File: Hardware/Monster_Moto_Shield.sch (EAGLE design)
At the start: 44 parts, among them Q1 FDD8580, Q2 FDD8580, U1 VNH2SP30, U2 VNH2SP30, U3 ARDUINO_SHIELDLABEL

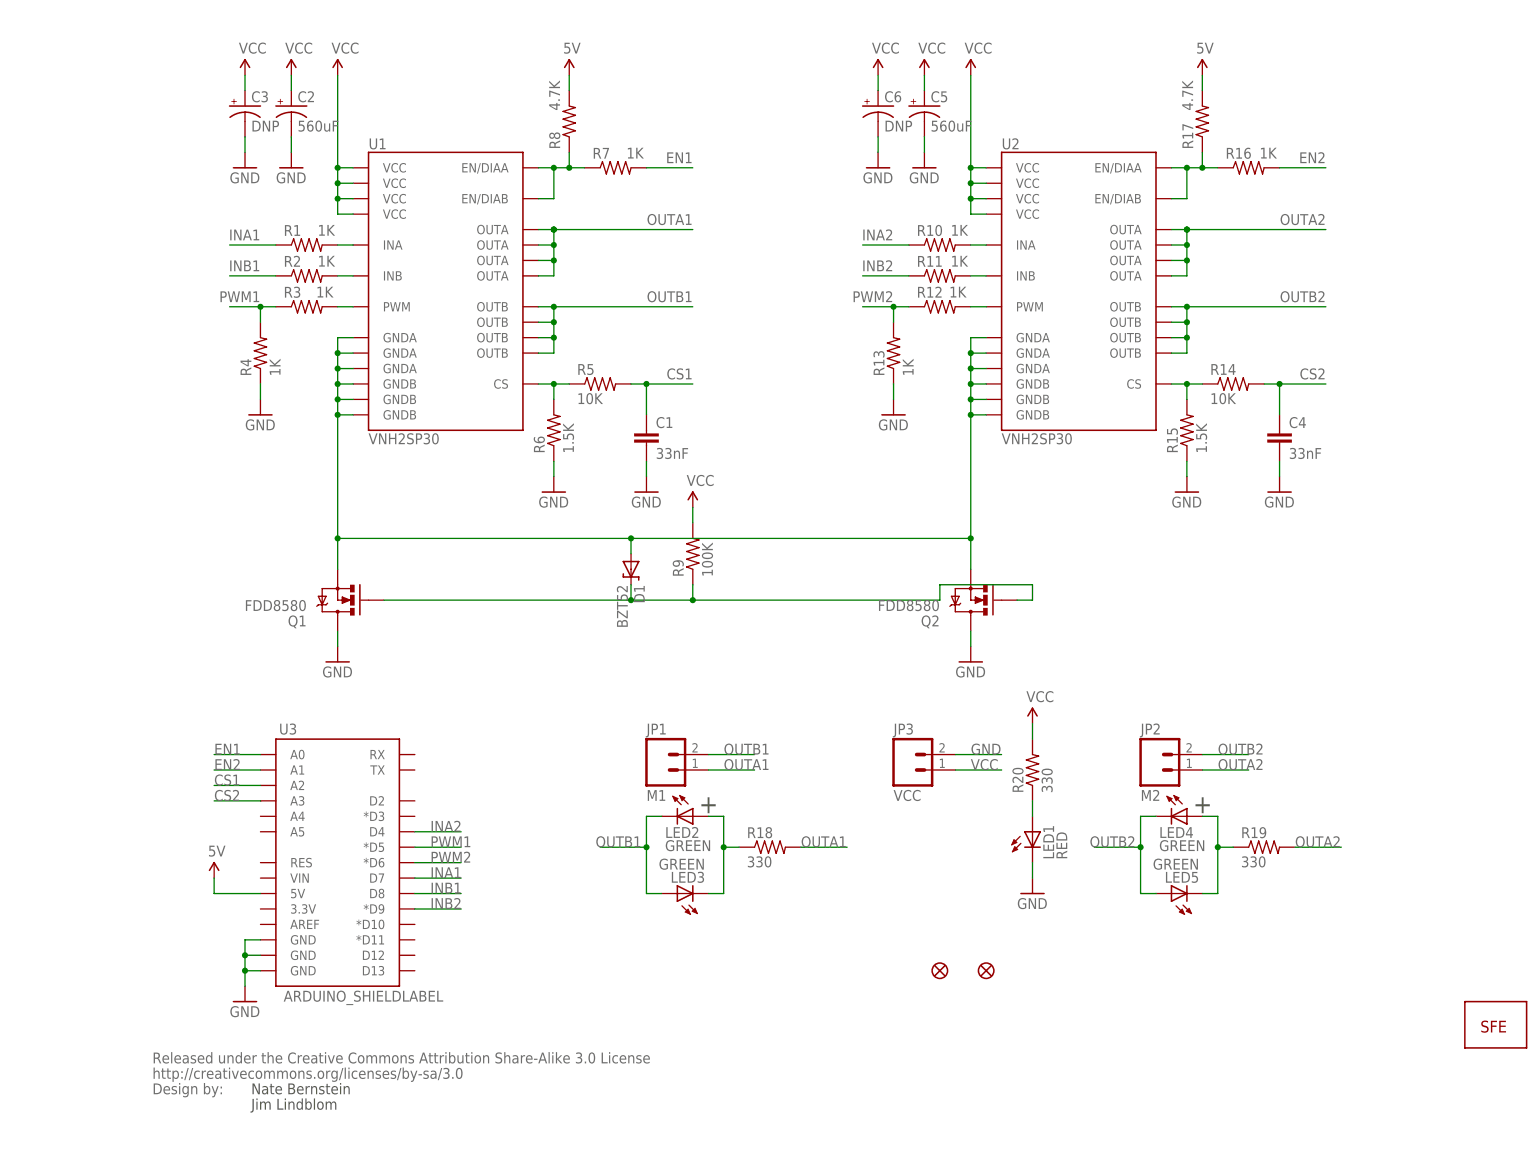
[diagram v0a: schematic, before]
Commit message: Commit bec of computer change
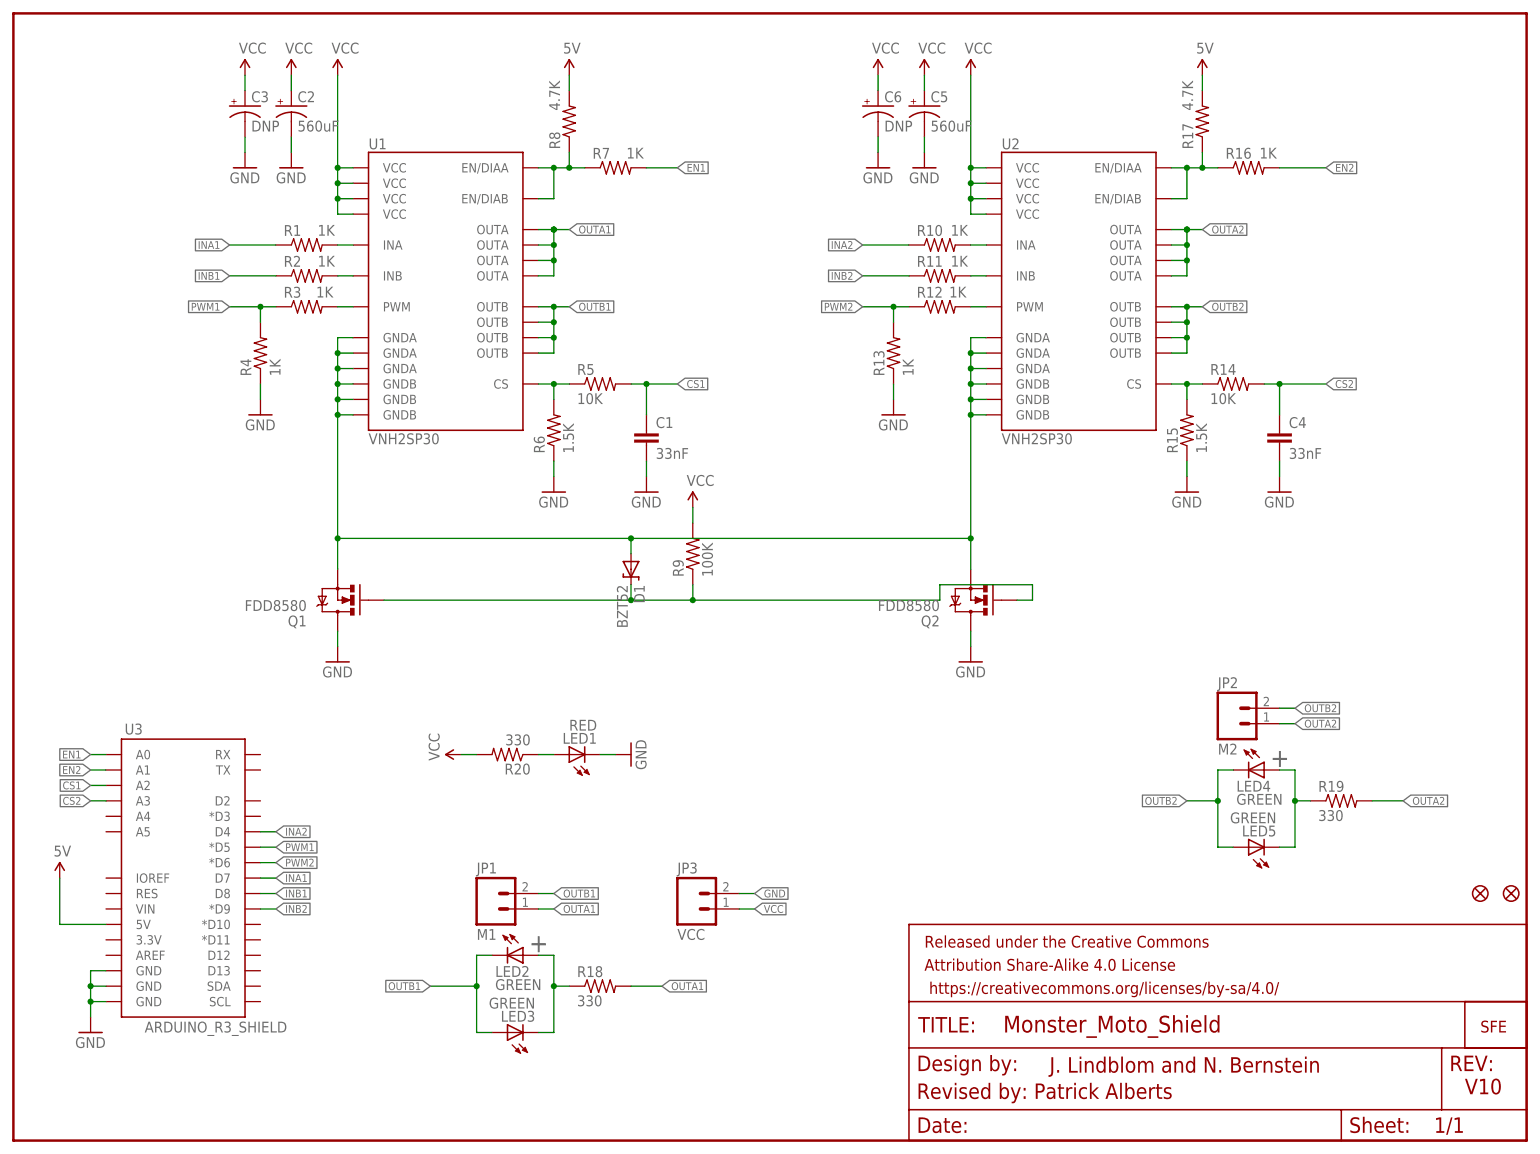
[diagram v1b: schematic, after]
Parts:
- removed U$6: CREATIVE_COMMONS, SparkFun:CREATIVE_COMMONS
- added FRAME*: FRAME-LETTER, SparkFun-Aesthetics:FRAME-LETTER
- U3: value ARDUINO_SHIELDLABEL -> ARDUINO_R3_SHIELD; device SparkFun:ARDUINO_SHIELDLABEL -> SparkFun-Boards:ARDUINO_R3_SHIELD
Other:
- note added: "J. Lindblom and N. Bernstein"
- note added: "Revised by: Patrick Alberts"
- note added: "V10"
- note removed: "Jim Lindblom"
- note removed: "Nate Bernstein"
- moved on the sheet: JP1, JP2, JP3, LED1, LED2, LED3, LED4, LED5, R18, R19, R20
